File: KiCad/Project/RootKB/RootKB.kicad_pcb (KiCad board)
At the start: 2 copper layers, 137.4 x 108.2 mm, 72 parts, among them J1 OLED-128x32, SW1 Switch, U1 Arduino_Pro_Micro, U2 TRRS

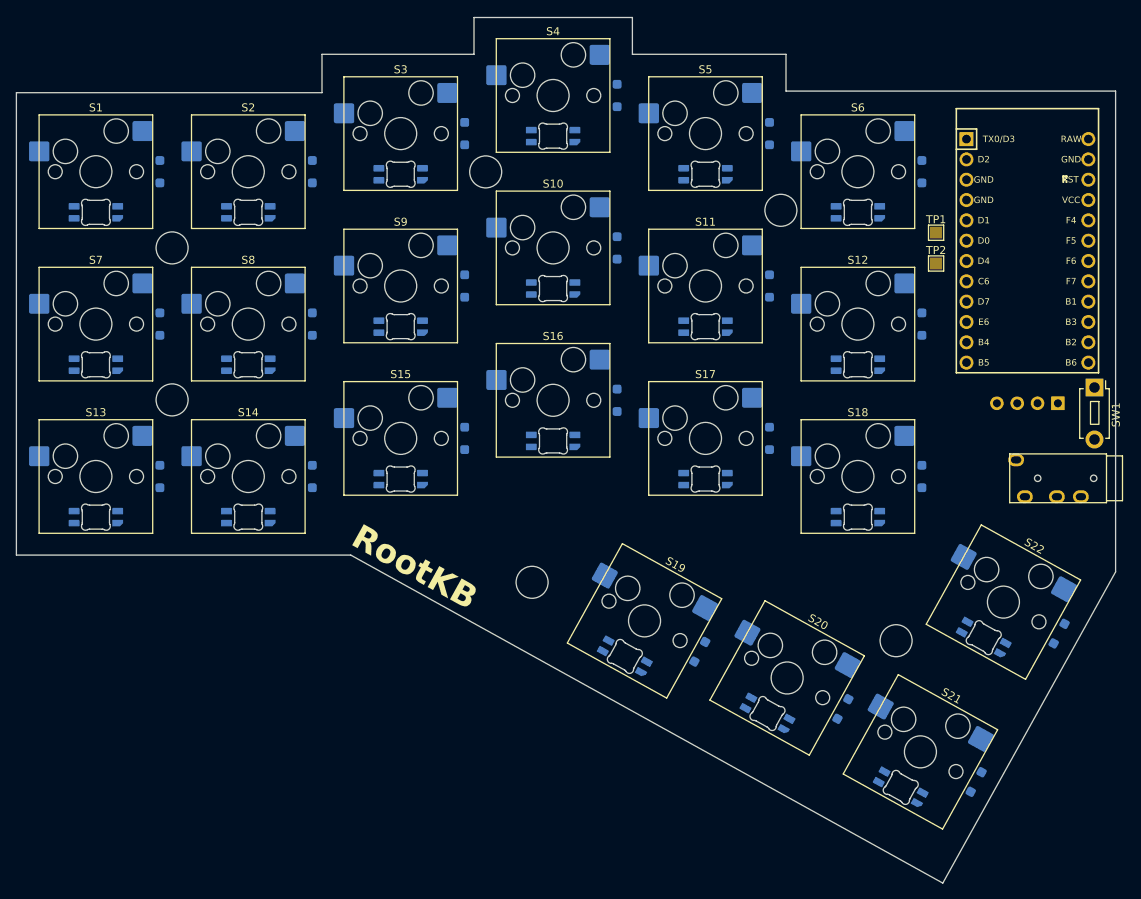
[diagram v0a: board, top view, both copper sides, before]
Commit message: update pcb
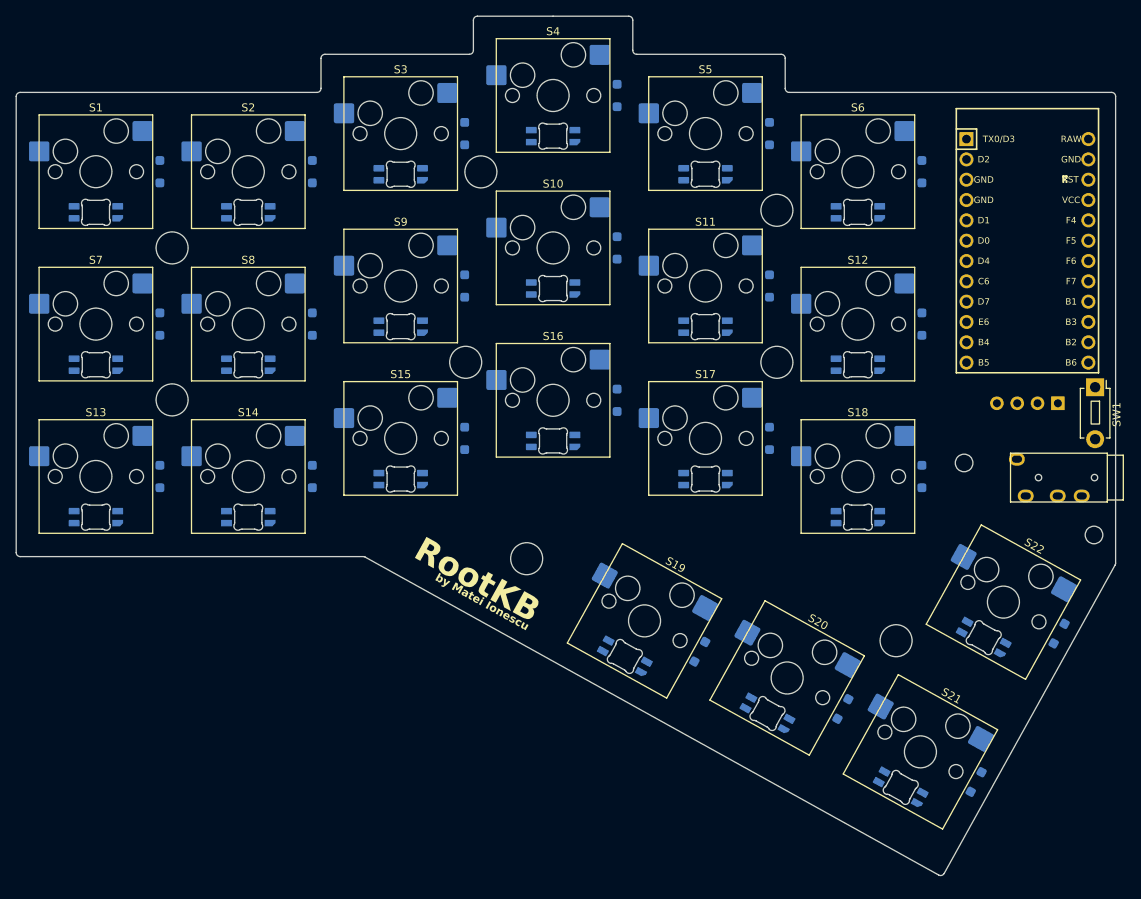
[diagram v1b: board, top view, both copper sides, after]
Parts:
- removed TP1, TP2: TestPoint, TestPoint:TestPoint_Pad_1.5x1.5mm
- moved U2 0.14 mm to (212.2, 100.1)
- moved SW1 0.09 mm to (210.6, 88.8)
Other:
- board size 137.4 x 108.2 mm -> 137.4 x 107.4 mm
- board text added: "by Matei Ionescu"
